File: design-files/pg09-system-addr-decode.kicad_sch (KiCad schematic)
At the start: 15 parts, among them U301 GAL22V10, U302 GAL22V10, U501 W65C21

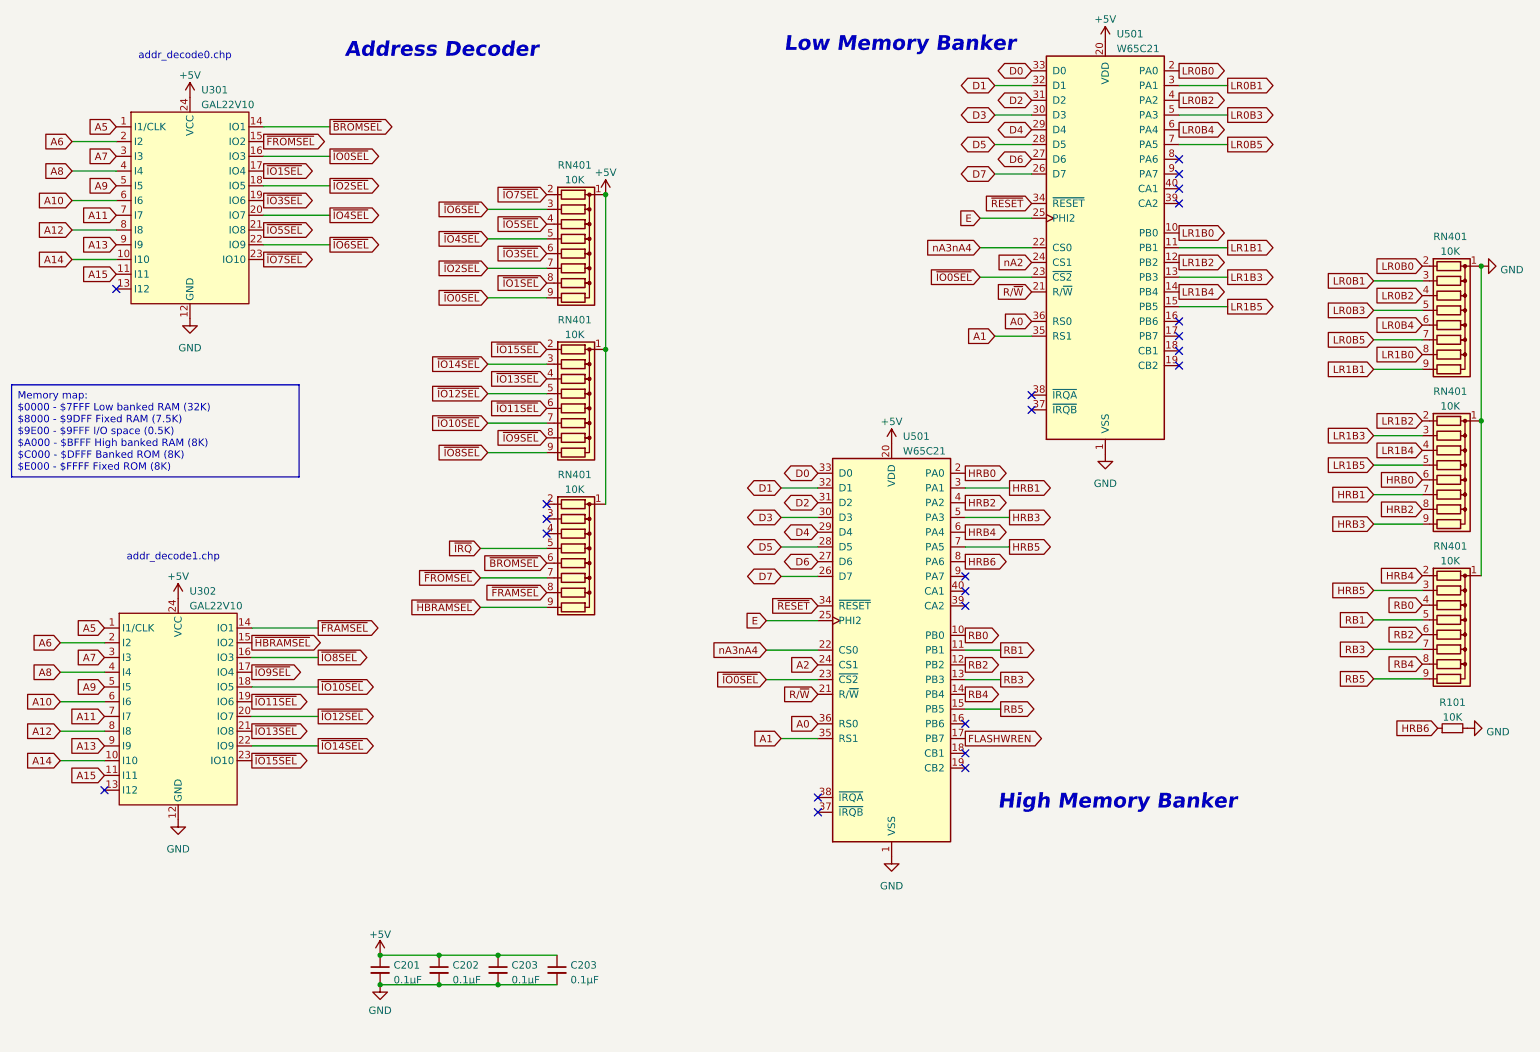
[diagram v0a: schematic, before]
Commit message: Move the misc system register decoder to the address decoder sheet.
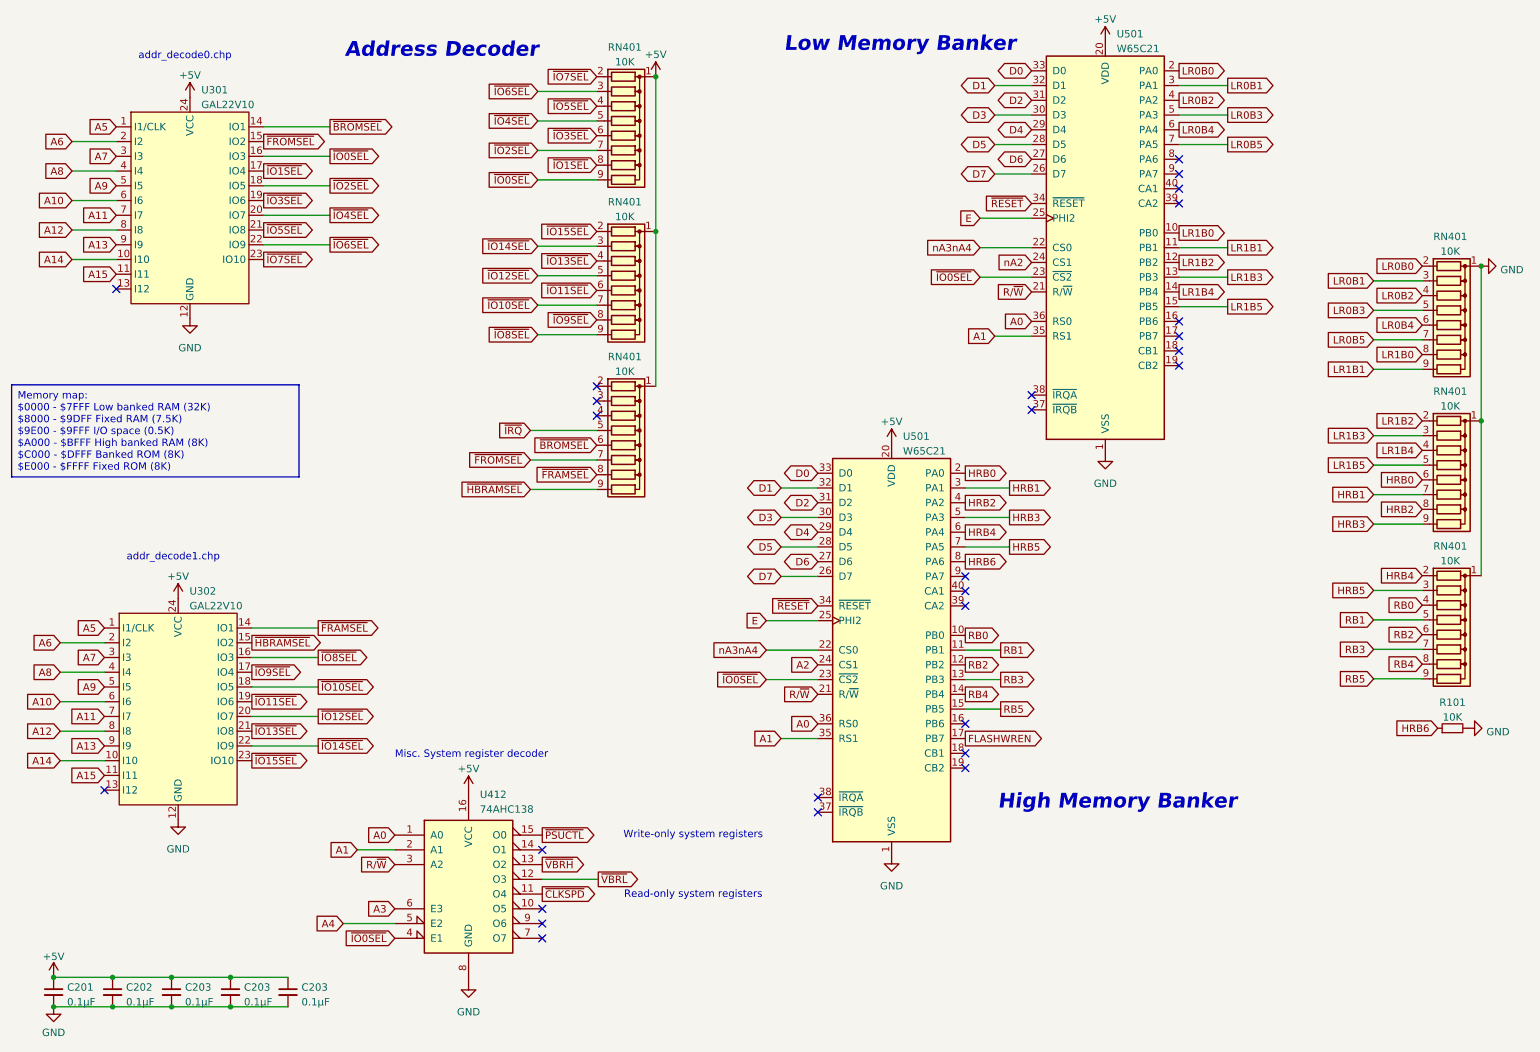
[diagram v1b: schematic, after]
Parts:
- added C203: 0.1µF, Capacitor_THT:C_Disc_D3.8mm_W2.6mm_P2.50mm, symbol Device:C_Small
- added U412: 74AHC138, Package_DIP:DIP-16_W7.62mm_Socket, symbol 74xx:74LS138
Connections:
- net +5V: now also C203.1, U412.16 (VCC)
- net A0: now also U412.1 (A0)
- net A1: now also U412.2 (A1)
- net GND: now also C203.2, U412.8 (GND)
- net R/~{W}: now also U412.3 (A2)
- net ~{IO0SEL}: now also U412.4 (E1)
- new net A3: U412.6 (E3)
- new net A4: U412.5 (E2)
- new net ~{CLKSPD}: U412.11 (O4)
- new net ~{PSUCTL}: U412.15 (O0)
- new net ~{VBRH}: U412.13 (O2)
- new net ~{VBRL}: U412.12 (O3)
- no-connect marks 23 -> 27
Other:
- note added: "Misc. System register decoder"
- note added: "Read-only system registers"
- note added: "Write-only system registers"
- moved on the sheet: C201, C202, C203, RN401
